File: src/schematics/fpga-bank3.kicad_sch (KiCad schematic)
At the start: 5 parts, among them U6 LFE5U-85F-*BG756*

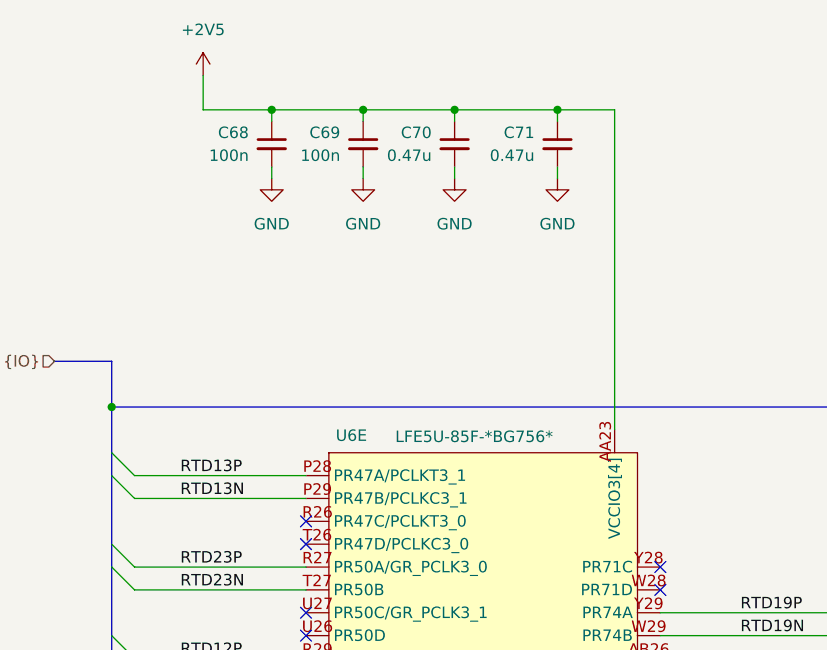
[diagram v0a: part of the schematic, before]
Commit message: Add bom components
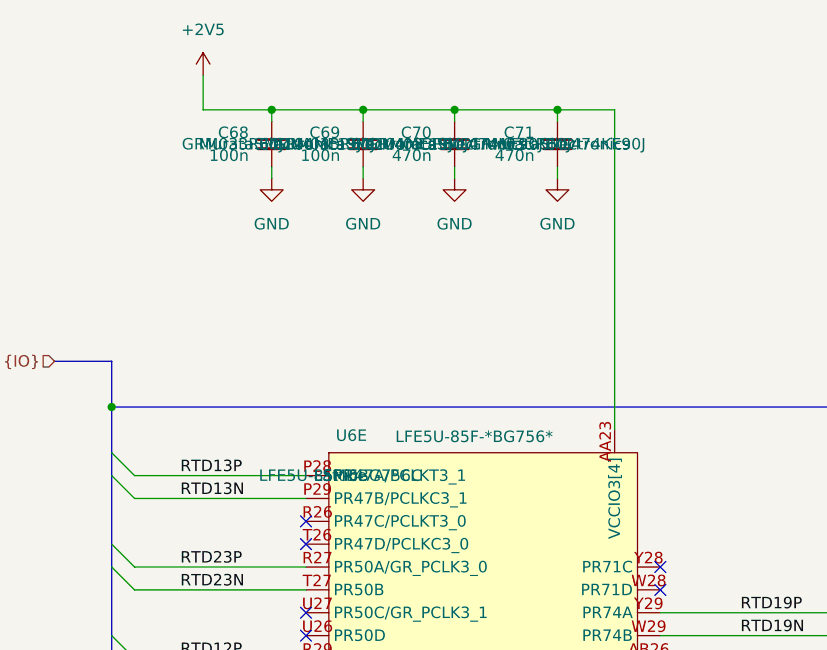
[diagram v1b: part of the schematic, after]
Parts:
- C68, C69: MPN (none) -> GRM033R60J104ME19J; Manufacturer (none) -> Murata Electronics; Mouting Technology (none) -> SMD
- C70, C71: value 0.47u -> 470n; MPN (none) -> GRM033R60J474KE90J; Manufacturer (none) -> Murata Electronics; Mouting Technology (none) -> SMD
- U6: MPN (none) -> LFE5U-85F-6BG756C; Manufacturer (none) -> Lattice; Mouting Technology (none) -> SMD
